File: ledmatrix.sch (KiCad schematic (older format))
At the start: 64 parts, among them U58 sled1735

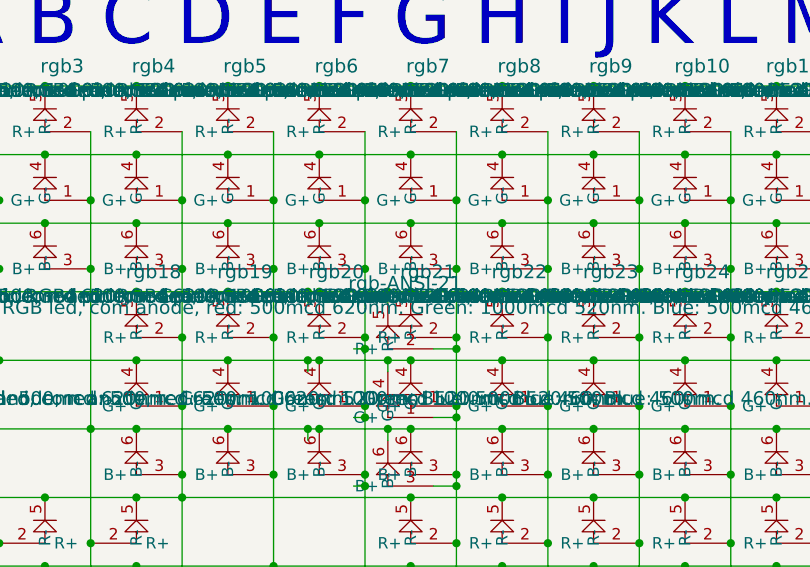
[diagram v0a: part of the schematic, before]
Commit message: post align
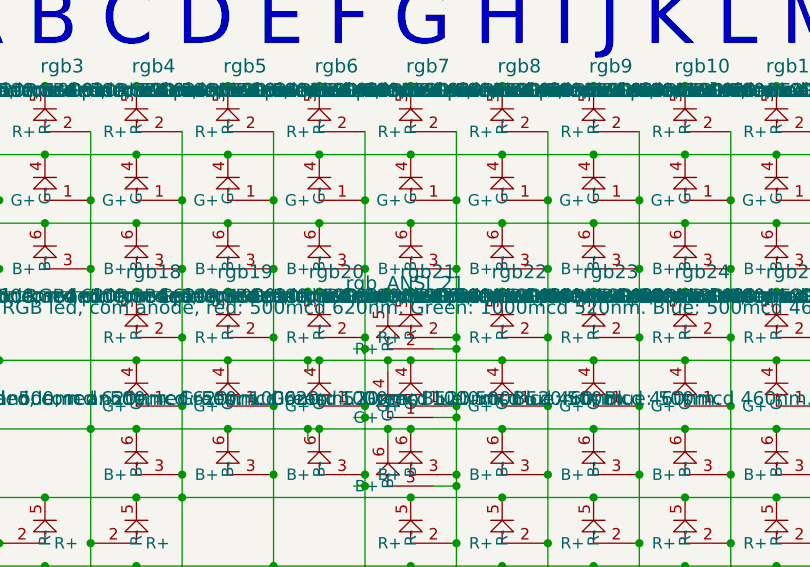
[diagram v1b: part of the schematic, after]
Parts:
- renumbered rgb-ANSI-21 to rgb_ANSI_21
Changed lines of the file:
@@
 $EndComp
 $Comp
-L rgbled rgb-ANSI-21
+L rgbled rgb_ANSI_21
 U 1 1 5AE32BA1
 P 4650 2450
-F 0 "rgb-ANSI-21" H 4725 3037 60  0000 C CNN
+F 0 "rgb_ANSI_21" H 4725 3037 60  0000 C CNN
 F 1 "4 pin RGB led, com anode, red: 500mcd 620nm. Green: 1000mcd 520nm. Blue: 500mcd 460nm." H 4725 2931 60  0000 C CNN
 F 2 "raise_fp:3528-4p-rev" H 4650 2450 60  0001 C CNN

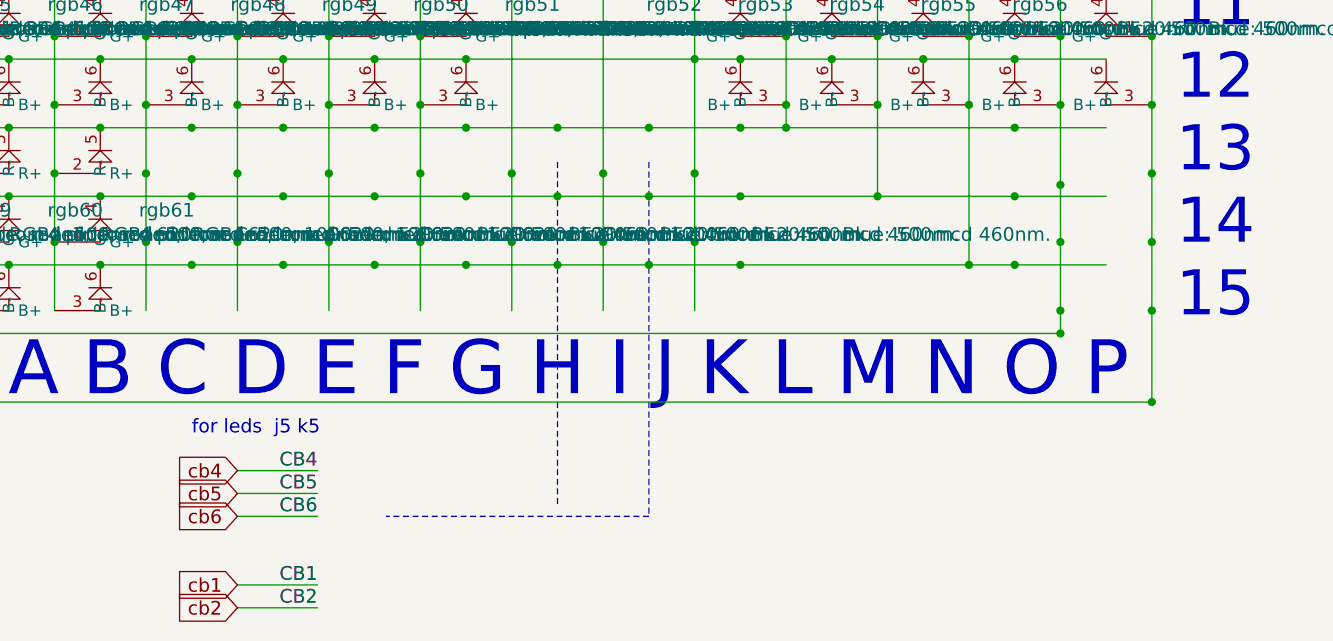
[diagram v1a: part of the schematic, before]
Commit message: new alignment
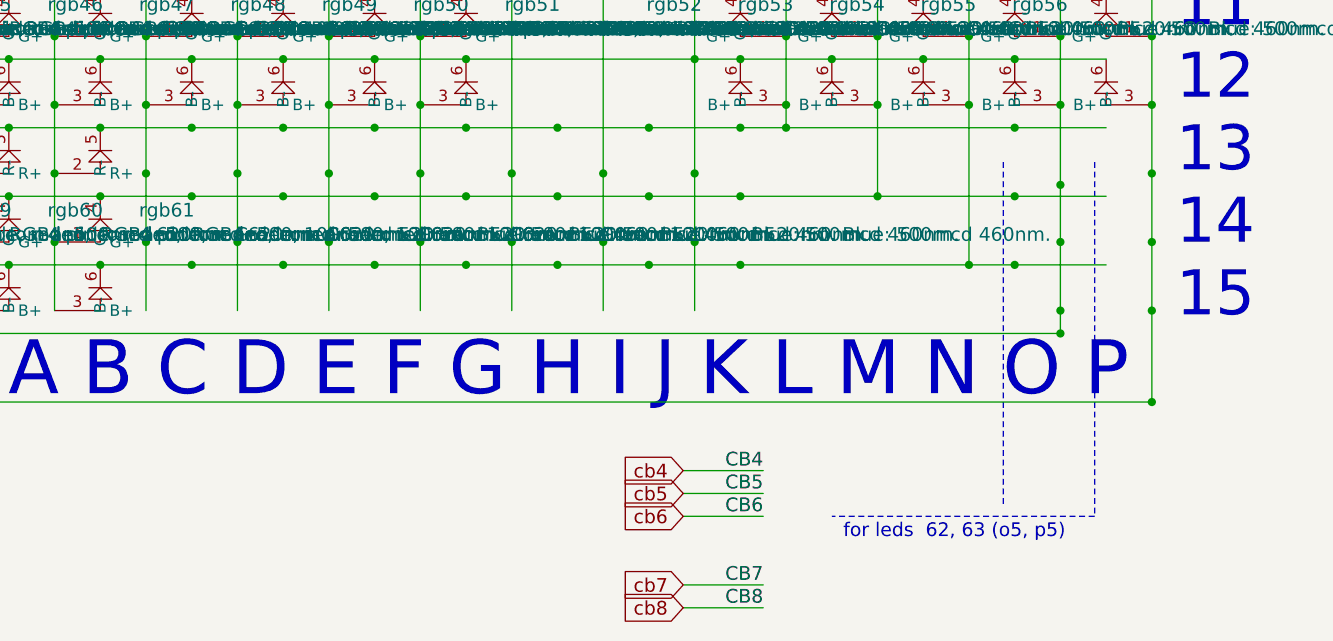
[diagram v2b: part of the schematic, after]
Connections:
- net labels added: cb7, cb8
- net labels removed: cb1, cb2
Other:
- note added: "for leds 62, 63 (o5, p5)\n\n"
- note removed: "for leds j5 k5"
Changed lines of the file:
@@
 Text Notes 2200 300  0    197  ~ 0
 common anode type 3 matrix
-Text Label 4100 6600 2    60   ~ 0
-CB1
-Text Label 4100 6700 2    60   ~ 0
-CB2
-Text Label 4100 6100 2    60   ~ 0
+Text Label 6050 6600 2    60   ~ 0
+CB7
+Text Label 6050 6700 2    60   ~ 0
+CB8
+Text Label 6050 6100 2    60   ~ 0
 CB4
-Text Label 4100 6200 2    60   ~ 0
+Text Label 6050 6200 2    60   ~ 0
 CB5
-Text Label 4100 6300 2    60   ~ 0
+Text Label 6050 6300 2    60   ~ 0
 CB6
 Wire Wire Line
-	4100 6100 3750 6100
+	6050 6100 5700 6100
 Wire Wire Line
-	3750 6200 4100 6200
+	5700 6200 6050 6200
 Wire Wire Line
-	4100 6300 3750 6300
+	6050 6300 5700 6300
 Wire Wire Line
-	4100 6600 3750 6600
+	6050 6600 5700 6600
 Wire Wire Line
-	3750 6700 4100 6700
+	5700 6700 6050 6700
 Text Notes 7650 850  2    236  ~ 0
 A B C D E F G H I J K L M N O P
@@
 Text Notes 750  5500 2    197  ~ 0
 1\n2\n3\n4\n5\n6\n7\n8\n9\n10\n11\n12\n13\n14\n15
-Text Notes 3550 5950 0    60   ~ 0
-for leds  j5 k5
-Text GLabel 3750 6100 0    60   Input ~ 0
+Text Notes 6400 6500 0    60   ~ 0
+for leds  62, 63 (o5, p5)\n\n
+Text GLabel 5700 6100 0    60   Input ~ 0
 cb4
-Text GLabel 3750 6200 0    60   Input ~ 0
+Text GLabel 5700 6200 0    60   Input ~ 0
 cb5
-Text GLabel 3750 6300 0    60   Input ~ 0
+Text GLabel 5700 6300 0    60   Input ~ 0
 cb6
-Text GLabel 3750 6600 0    60   Input ~ 0
-cb1
-Text GLabel 3750 6700 0    60   Input ~ 0
-cb2
+Text GLabel 5700 6600 0    60   Input ~ 0
+cb7
+Text GLabel 5700 6700 0    60   Input ~ 0
+cb8
 $Comp
 L Earth #PWR031
@@
 $EndComp
 Wire Notes Line
-	5550 4750 5550 6300
+	7500 4750 7500 6300
 Wire Notes Line
-	5550 6300 4400 6300
+	7500 6300 6350 6300
 Wire Notes Line
-	5150 4750 5150 6250
+	7100 4750 7100 6250
 $Comp
 L rgbled rgb1
